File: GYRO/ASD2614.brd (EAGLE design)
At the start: 22.5 x 21.3 mm, 25 parts, among them J1 3013, J2 DF12-32-DP, J3 961102, J4 SM02B-SRSS-TB(LF)(SN), Q2 DMP2035U, SW1 PCM12SMTR, U1 ATMEGA328P, U2 MCP73831, Y1 8.00MHZ

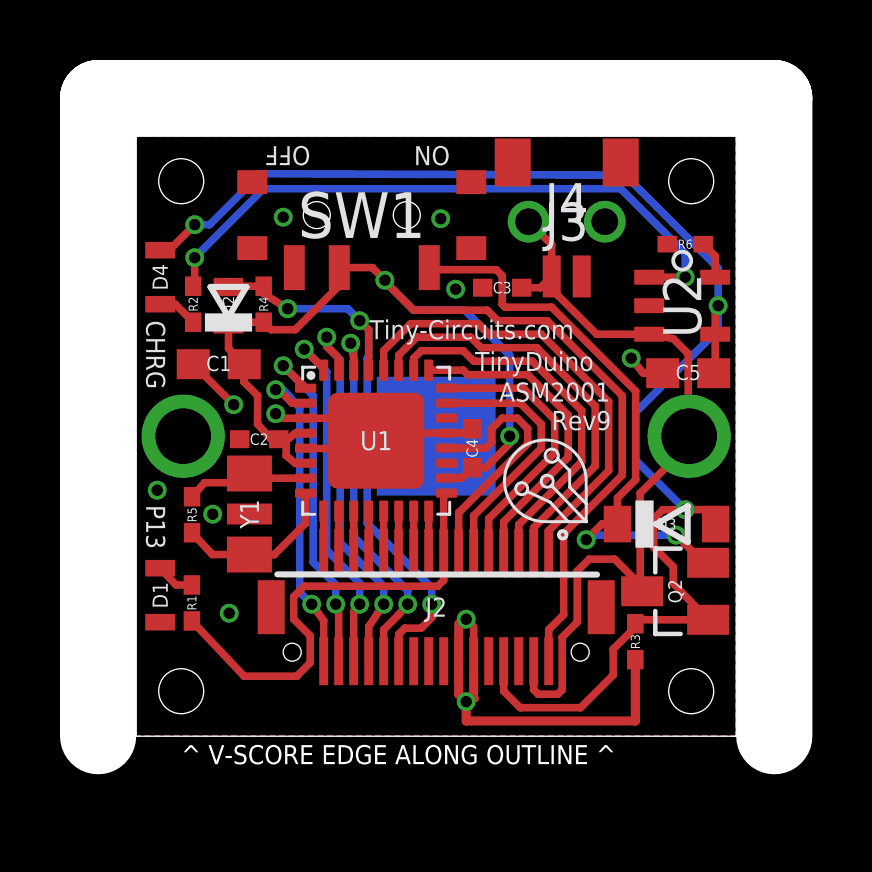
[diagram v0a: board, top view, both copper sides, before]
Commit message: asdsa
asd
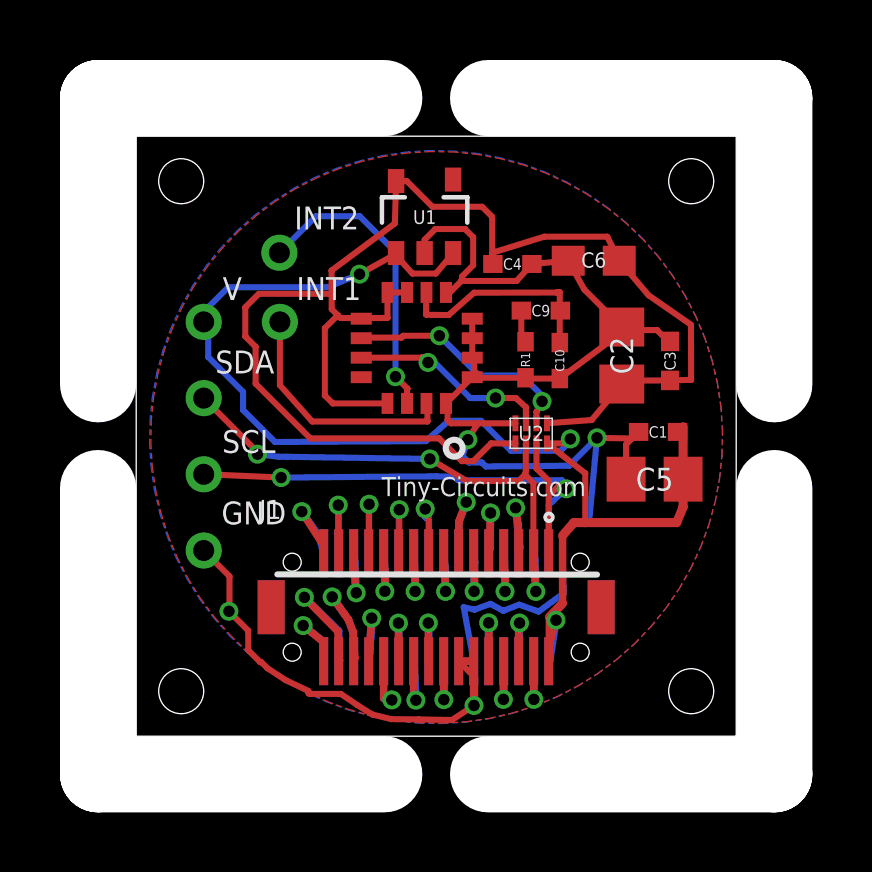
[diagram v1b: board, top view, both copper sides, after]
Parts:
- removed D1: GREEN, tinycircuits:LNJ_LED
- removed D2: CD0603, tinycircuits:0603
- removed D3: MBR120, tinycircuits:SOD-123FL
- removed D4: AMBER, tinycircuits:LNJ_LED
- removed Q2: DMP2035U, tinycircuits:SOT23
- removed R2: 1k, tinycircuits:0402
- removed R3: 100k, tinycircuits:0402
- removed R4, R6: 10K, tinycircuits:0402
- removed R5: 1M, tinycircuits:0402
- removed SW1: PCM12SMTR, tinycircuits:PCM12SMTR
- removed Y1: 8.00MHZ, tinycircuits:RESONATOR_SMALL
- added C10: 10nF, tinycircuits:0402
- added C6: 10uF, tinycircuits:C0603
- added C9: 0.47uF, tinycircuits:C0402
- added J5, J6, J7, J8: PIN_1X.1", tinycircuits:1X.1"
- added U4: L3G4200D, tinycircuits:L3G4200D
- C1: value 10uF -> 0.1uF; device tinycircuits:C0603 -> tinycircuits:C0402
- C2: value .1uF -> 10uF; device tinycircuits:C0402 -> tinycircuits:C0805
- C3: value 4.7uF -> 0.1uF
- C4: value .1uF -> 0.1uF
- C5: device tinycircuits:C0603 -> tinycircuits:C0805
- J1: value 3013 -> DF12-32-DP; device tinycircuits:3013 -> tinycircuits:DF12-32-DP
- J2: value DF12-32-DP -> DF12-32-DS; device tinycircuits:DF12-32-DP -> tinycircuits:DF12-32-DS
- J3: value 961102 -> PIN_1X.1"; device tinycircuits:2X.1" -> tinycircuits:1X.1"
- J4: value SM02B-SRSS-TB(LF)(SN) -> PIN_1X.1"; device tinycircuits:JST_SH_2X1 -> tinycircuits:1X.1"
- R1: value 1k -> 10.0K
- U1: value ATMEGA328P -> XC6210B33; device tinycircuits:ATMEL_QFN32 -> tinycircuits:SOT-25
- U2: value MCP73831 -> TX0102; device tinycircuits:SOT-23 -> tinycircuits:DQE(R-PX2SON-N8)
- moved C1 14.8 mm to (27.4, 20.1)
- moved R1 13.8 mm to (23.0, 22.5)
- moved J4 13.7 mm to (12.2, 21.3), turned to 0 degrees
- moved J3 12.6 mm to (12.2, 23.8)
- moved C2 12.4 mm to (26.2, 22.7), turned to 90 degrees
- moved U1 7.63 mm to (19.6, 27.3)
- moved U2 6.59 mm to (23.2, 20.1), turned to 180 degrees
- moved C4 6.29 mm to (22.5, 25.7), turned to 0 degrees
- moved C3 6.10 mm to (27.8, 22.5), turned to 90 degrees
- moved J1 5.70 mm to (20.0, 14.3), flipped to the top, turned to 180 degrees
- moved C5 3.71 mm to (27.3, 18.6)
- moved U$1 0.09 mm to (43.9, 0.00)
- flipped J2 to the bottom, turned to 0 degrees
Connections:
- removed net 1: J1.1
- removed net N$3: R5.1, U1.7, Y1.3
- removed net N$4: D1.A, R1.1
- removed net N$5: D4.C, R2.1
- removed net N$6: R6.1, U2.5
- removed net N$7: R2.2, U2.1
- new net INT1: J7.1, U4.7
- new net INT2: J8.1, U4.6
- new net SCL_3V3: U2.2, U4.2
- new net SDA_3V3: U2.3, U4.3
- new net VCC_3V3: C2.1, C3.1, C4.1, C6.1, U1.5, U2.1, U2.5, U4.1, U4.15, U4.16, U4.5
- net +3V3: now also J1.6
- net +5V: now also J1.8; no longer C5.1, D3.A, D4.A, Q2.B, R3.2, U2.4
- net AD0: now also J1.11; no longer U1.23
- net AD1: now also J1.9; no longer U1.24
- net AD2: now also J1.7; no longer U1.25
- net AD3: now also J1.5; no longer U1.26
- net AD4/SDA: now also J1.3, J4.1, U2.6; no longer U1.27
- net AD5/SCL: now also J1.1, J5.1, U2.7; no longer U1.28
- net AREF: now also J1.13; no longer U1.20
- net GND: now also C10.2, C6.2, J1.12, J1.14, J6.1, R1.2, U1.2, U2.4, U4.10, U4.11, U4.12, U4.13, U4.8, U4.9; no longer D1.C, J1.3, J3.2, J4.1, R3.1, R6.2, SW1.W1, SW1.W2, SW1.W3, SW1.W4, U1.21, U1.3, U1.5, U1.EXP, U2.2, Y1.2
- net IO0: now also J1.24; no longer U1.30
- net IO1: now also J1.26; no longer U1.31
- net IO2: now also J1.28; no longer U1.32
- net IO3: now also J1.30; no longer U1.1
- net IO4: now also J1.32; no longer U1.2
- net IO5: now also J1.31; no longer U1.9
- net IO6: now also J1.29; no longer U1.10
- net IO7: now also J1.27; no longer U1.11
- net IO8: now also J1.25; no longer U1.12
- net IO9: now also J1.23; no longer U1.13
- net MISO: now also J1.17; no longer U1.16
- net MOSI: now also J1.19; no longer U1.15
- net N$1: now also C9.2, R1.1; no longer R5.2, U1.8, Y1.1
- net N$2: now also C10.1, C9.1, U4.14; no longer D3.C, Q2.E, SW1.1
- net RESET: now also J1.22; no longer D2.A, R4.1, U1.29
- net RSV0: now also J1.20
- net RSV1: now also J1.18
- net RSV2: now also J1.16
- net SCK: now also J1.15; no longer R1.2, U1.17
- net SS: now also J1.21; no longer U1.14
- net VBATT: now also J1.4; no longer C3.1, J1.2, J3.1, J4.2, Q2.C, U2.3
- net VCC: now also C5.1, J1.2, J3.1, U1.1, U1.3, U2.8; no longer C2.1, C4.1, D2.C, R4.2, SW1.2, U1.18, U1.4, U1.6
- net VIN: now also J1.10
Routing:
- net VCC_3V3: track 0.00 -> 50.8 mm
- net +5V: track 49.9 -> 2.58 mm, vias 3 -> 1
- net GND: track 28.5 -> 65.4 mm, vias 11 -> 4
- net VBATT: track 26.7 -> 2.55 mm, vias 0 -> 1
- net N$7: track 21.2 -> 0.00 mm, vias 2 -> 0
- net RESET: track 20.1 -> 2.55 mm, vias 3 -> 1
- net SCK: track 15.5 -> 2.55 mm, vias 0 -> 1
- net N$2: track 19.6 -> 7.26 mm, vias 2 -> 0
- net INT2: track 0.00 -> 10.1 mm, vias 0 -> 1
- net IO0: track 12.6 -> 3.06 mm, vias 2 -> 1
- net AD3: track 12.6 -> 3.04 mm, vias 0 -> 1
- net IO1: track 13.0 -> 4.07 mm, vias 2 -> 1
- net INT1: track 0.00 -> 8.37 mm
- net AD2: track 10.8 -> 2.55 mm, vias 0 -> 1
- net IO4: track 11.0 -> 3.04 mm, vias 2 -> 1
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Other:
- board size 22.5 x 21.3 mm -> 22.5 x 22.5 mm
- board text added: "1"
- board text added: "3-Axis Gyro"
- board text added: "AS-PCB-ASD2614"
- board text added: "ASD2614 - Rev1"
- board text added: "GND"
- board text added: "INT1"
- board text added: "INT2"
- board text added: "R1"
- board text added: "R2"
- board text added: "SCL"
- board text added: "SDA"
- board text added: "TinyShield - 3-Axis Gyro"
- board text added: "V"
- board text removed: "+"
- board text removed: "-"
- board text removed: "9"
- board text removed: "AS-PCB-ASM2001"
- board text removed: "ASM2001"
- board text removed: "CHRG"
- board text removed: "OFF"
- board text removed: "ON"
- board text removed: "P13"
- board text removed: "Rev9"
- board text removed: "TinyDuino"
- board text removed: "TinyDuino - 20mm"
- board text removed: "^ V-SCORE EDGE ALONG OUTLINE ^"
